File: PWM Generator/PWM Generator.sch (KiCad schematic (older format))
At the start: 8 parts

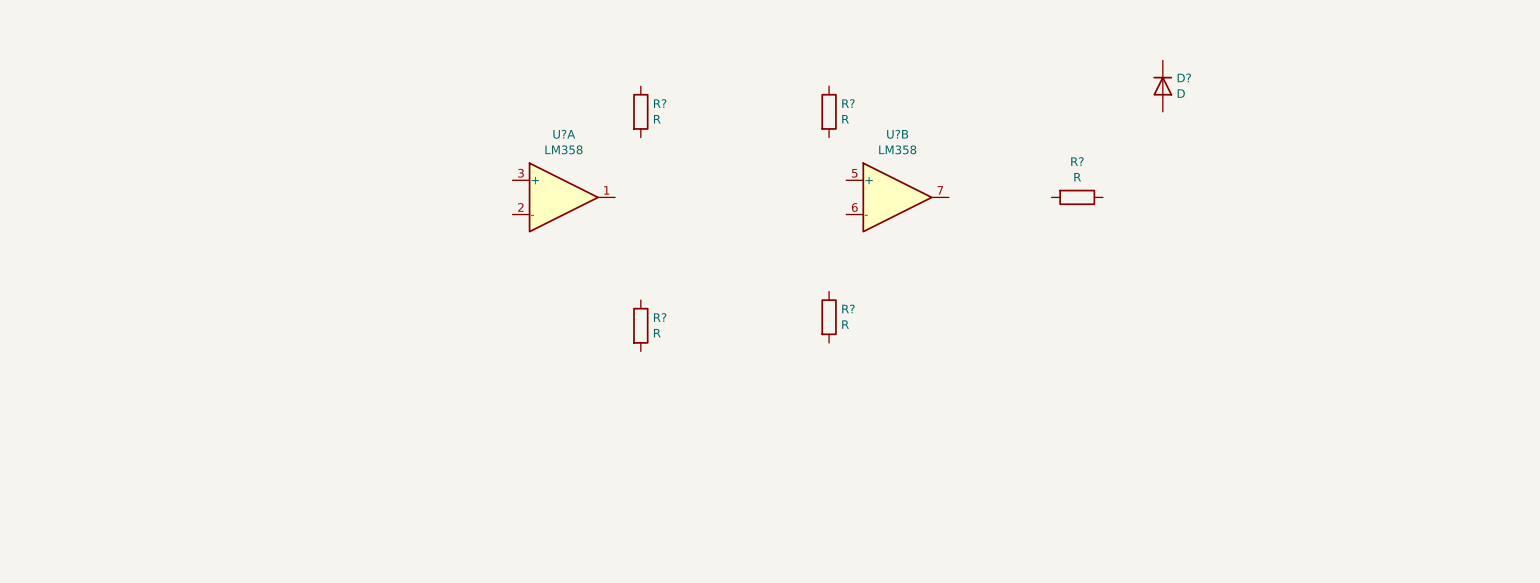
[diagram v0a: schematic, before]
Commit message: wired connection
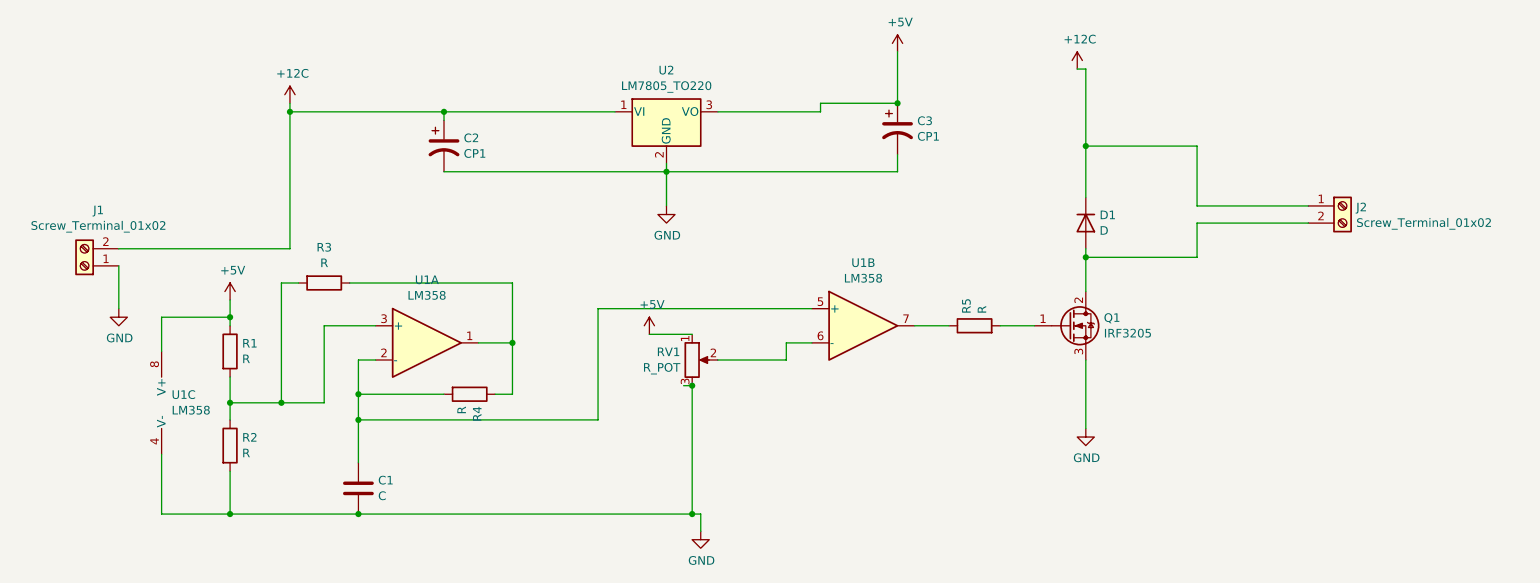
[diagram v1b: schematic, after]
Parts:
- added C1: C, symbol Device:C
- added C2, C3: CP1, symbol Device:CP1
- added J1, J2: Screw_Terminal_01x02, symbol Connector:Screw_Terminal_01x02
- added Q1: IRF3205, Package_TO_SOT_THT:TO-220-3_Vertical, symbol Transistor_FET:IRF3205
- added RV1: R_POT, symbol Device:R_POT
- added unit 3 of U1
- added U2: LM7805_TO220, Package_TO_SOT_THT:TO-220-3_Vertical, symbol Regulator_Linear:LM7805_TO220
- gave numbers to parts that had none: 7
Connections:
- net at U1.1: now also R3.1, R4.1
- net at U1.2 (-): now also R4.2, U1.5 (+), C1.1
- net at U1.3 (+): now also R1.2, R2.1, R3.2
- net at U1.6 (-): now also RV1.2
- net at U1.7: now also R5.1
- net +12C: now reaches D1.1 (K)
- net +12C: now also C2.1, J1.2 (Pin_2), J2.1 (Pin_1), U2.1 (VI)
- net at D1.2 (A): now also J2.2 (Pin_2), Q1.2 (D)
- net +5V: now reaches R1.1
- net +5V: now also C3.1, RV1.1, U1.8 (V+), U2.3 (VO)
- net GND: now reaches R2.2
- net GND: now also C1.2, C2.2, C3.2, J1.1 (Pin_1), Q1.3 (S), RV1.3, U1.4 (V-), U2.2 (GND)
- net at R5.2: now also Q1.1 (G)
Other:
- moved on the sheet: D1, R1, R2, R3, R4, R5, U1A, U1B

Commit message: PCB net
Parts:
- C1: footprint (none) -> Capacitor_THT:C_Radial_D6.3mm_H5.0mm_P2.50mm
- C2: footprint (none) -> Capacitor_THT:CP_Radial_D10.0mm_P3.50mm
- C3: footprint (none) -> Capacitor_THT:CP_Radial_D7.5mm_P2.50mm
- D1: footprint (none) -> Diode_THT:D_DO-27_P15.24mm_Horizontal
- J1, J2: footprint (none) -> TerminalBlock_4Ucon:TerminalBlock_4Ucon_1x02_P3.50mm_Horizontal
- R1: footprint (none) -> Resistor_THT:R_Radial_Power_L16.1mm_W9.0mm_P7.37mm
- R2, R4, R5: footprint (none) -> Resistor_THT:R_Radial_Power_L11.0mm_W7.0mm_P5.00mm
- R3: footprint (none) -> Resistor_THT:R_Radial_Power_L13.0mm_W9.0mm_P5.00mm
- RV1: footprint (none) -> Potentiometer_THT:Potentiometer_Runtron_RM-065_Vertical
- U1: footprint (none) -> Package_DIP:DIP-8_W7.62mm
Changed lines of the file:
@@
 F 0 "U1" H 3600 2867 50  0000 C CNN
 F 1 "LM358" H 3600 2776 50  0000 C CNN
-F 2 "" H 3600 2500 50  0001 C CNN
+F 2 "Package_DIP:DIP-8_W7.62mm" H 3600 2500 50  0001 C CNN
 F 3 "http://www.ti.com/lit/ds/symlink/lm2904-n.pdf" H 3600 2500 50  0001 C CNN
 	1    3600 2500
@@
 F 0 "U1" H 6150 2767 50  0000 C CNN
 F 1 "LM358" H 6150 2676 50  0000 C CNN
-F 2 "" H 6150 2400 50  0001 C CNN
+F 2 "Package_DIP:DIP-8_W7.62mm" H 6150 2400 50  0001 C CNN
 F 3 "http://www.ti.com/lit/ds/symlink/lm2904-n.pdf" H 6150 2400 50  0001 C CNN
 	2    6150 2400
@@
 F 0 "R4" H 3920 2846 50  0000 L CNN
 F 1 "R" H 3920 2755 50  0000 L CNN
-F 2 "" V 3780 2800 50  0001 C CNN
+F 2 "Resistor_THT:R_Radial_Power_L11.0mm_W7.0mm_P5.00mm" V 3780 2800 50  0001 C CNN
 F 3 "~" H 3850 2800 50  0001 C CNN
 	1    3850 2800
@@
 F 0 "R1" H 2520 2596 50  0000 L CNN
 F 1 "R" H 2520 2505 50  0000 L CNN
-F 2 "" V 2380 2550 50  0001 C CNN
+F 2 "Resistor_THT:R_Radial_Power_L16.1mm_W9.0mm_P7.37mm" V 2380 2550 50  0001 C CNN
 F 3 "~" H 2450 2550 50  0001 C CNN
 	1    2450 2550
@@
 F 0 "R2" H 2520 3146 50  0000 L CNN
 F 1 "R" H 2520 3055 50  0000 L CNN
-F 2 "" V 2380 3100 50  0001 C CNN
+F 2 "Resistor_THT:R_Radial_Power_L11.0mm_W7.0mm_P5.00mm" V 2380 3100 50  0001 C CNN
 F 3 "~" H 2450 3100 50  0001 C CNN
 	1    2450 3100
@@
 F 0 "R5" H 6870 2446 50  0000 L CNN
 F 1 "R" H 6870 2355 50  0000 L CNN
-F 2 "" V 6730 2400 50  0001 C CNN
+F 2 "Resistor_THT:R_Radial_Power_L11.0mm_W7.0mm_P5.00mm" V 6730 2400 50  0001 C CNN
 F 3 "~" H 6800 2400 50  0001 C CNN
 	1    6800 2400
@@
 F 0 "R3" V 2793 2150 50  0000 C CNN
 F 1 "R" V 2884 2150 50  0000 C CNN
-F 2 "" V 2930 2150 50  0001 C CNN
+F 2 "Resistor_THT:R_Radial_Power_L13.0mm_W9.0mm_P5.00mm" V 2930 2150 50  0001 C CNN
 F 3 "~" H 3000 2150 50  0001 C CNN
 	1    3000 2150
@@
 F 0 "D1" V 7404 1880 50  0000 L CNN
 F 1 "D" V 7495 1880 50  0000 L CNN
-F 2 "" H 7450 1800 50  0001 C CNN
+F 2 "Diode_THT:D_DO-27_P15.24mm_Horizontal" H 7450 1800 50  0001 C CNN
 F 3 "~" H 7450 1800 50  0001 C CNN
 	1    7450 1800
@@
 F 0 "C1" H 3315 3396 50  0000 L CNN
 F 1 "C" H 3315 3305 50  0000 L CNN
-F 2 "" H 3238 3200 50  0001 C CNN
+F 2 "Capacitor_THT:C_Radial_D6.3mm_H5.0mm_P2.50mm" H 3238 3200 50  0001 C CNN
 F 3 "~" H 3200 3350 50  0001 C CNN
 	1    3200 3350
@@
 F 0 "C2" H 3815 1396 50  0000 L CNN
 F 1 "CP1" H 3815 1305 50  0000 L CNN
-F 2 "" H 3700 1350 50  0001 C CNN
+F 2 "Capacitor_THT:CP_Radial_D10.0mm_P3.50mm" H 3700 1350 50  0001 C CNN
 F 3 "~" H 3700 1350 50  0001 C CNN
 	1    3700 1350
@@
 F 0 "C3" H 6465 1296 50  0000 L CNN
 F 1 "CP1" H 6465 1205 50  0000 L CNN
-F 2 "" H 6350 1250 50  0001 C CNN
+F 2 "Capacitor_THT:CP_Radial_D7.5mm_P2.50mm" H 6350 1250 50  0001 C CNN
 F 3 "~" H 6350 1250 50  0001 C CNN
 	1    6350 1250
@@
 F 0 "J2" H 9030 1692 50  0000 L CNN
 F 1 "Screw_Terminal_01x02" H 9030 1601 50  0000 L CNN
-F 2 "" H 8950 1700 50  0001 C CNN
+F 2 "TerminalBlock_4Ucon:TerminalBlock_4Ucon_1x02_P3.50mm_Horizontal" H 8950 1700 50  0001 C CNN
 F 3 "~" H 8950 1700 50  0001 C CNN
 	1    8950 1700
@@
 F 0 "J1" H 1518 1725 50  0000 C CNN
 F 1 "Screw_Terminal_01x02" H 1518 1816 50  0000 C CNN
-F 2 "" H 1600 2050 50  0001 C CNN
+F 2 "TerminalBlock_4Ucon:TerminalBlock_4Ucon_1x02_P3.50mm_Horizontal" H 1600 2050 50  0001 C CNN
 F 3 "~" H 1600 2050 50  0001 C CNN
 	1    1600 2050
@@
 F 0 "RV1" H 5081 2646 50  0000 R CNN
 F 1 "R_POT" H 5081 2555 50  0000 R CNN
-F 2 "" H 5150 2600 50  0001 C CNN
+F 2 "Potentiometer_THT:Potentiometer_Runtron_RM-065_Vertical" H 5150 2600 50  0001 C CNN
 F 3 "~" H 5150 2600 50  0001 C CNN
 	1    5150 2600
@@
 F 0 "U1" H 2108 2896 50  0000 L CNN
 F 1 "LM358" H 2108 2805 50  0000 L CNN
-F 2 "" H 2150 2850 50  0001 C CNN
+F 2 "Package_DIP:DIP-8_W7.62mm" H 2150 2850 50  0001 C CNN
 F 3 "http://www.ti.com/lit/ds/symlink/lm2904-n.pdf" H 2150 2850 50  0001 C CNN
 	3    2150 2850
